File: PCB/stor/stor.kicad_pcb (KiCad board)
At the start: 4 copper layers, 22 x 60.5 mm, 55 parts, among them J1 Conn_01x05_Socket, J2 Conn_01x04_Socket, SW1 TS1603-TZ38HBM, SW2 TS1603-TZ38HBM, U1 STM32H723VGT6, U3 USB3300-EZK-TR, U4 TPS62177DQCR, X1 25mhz, X2 32.768k, X3 24mhz

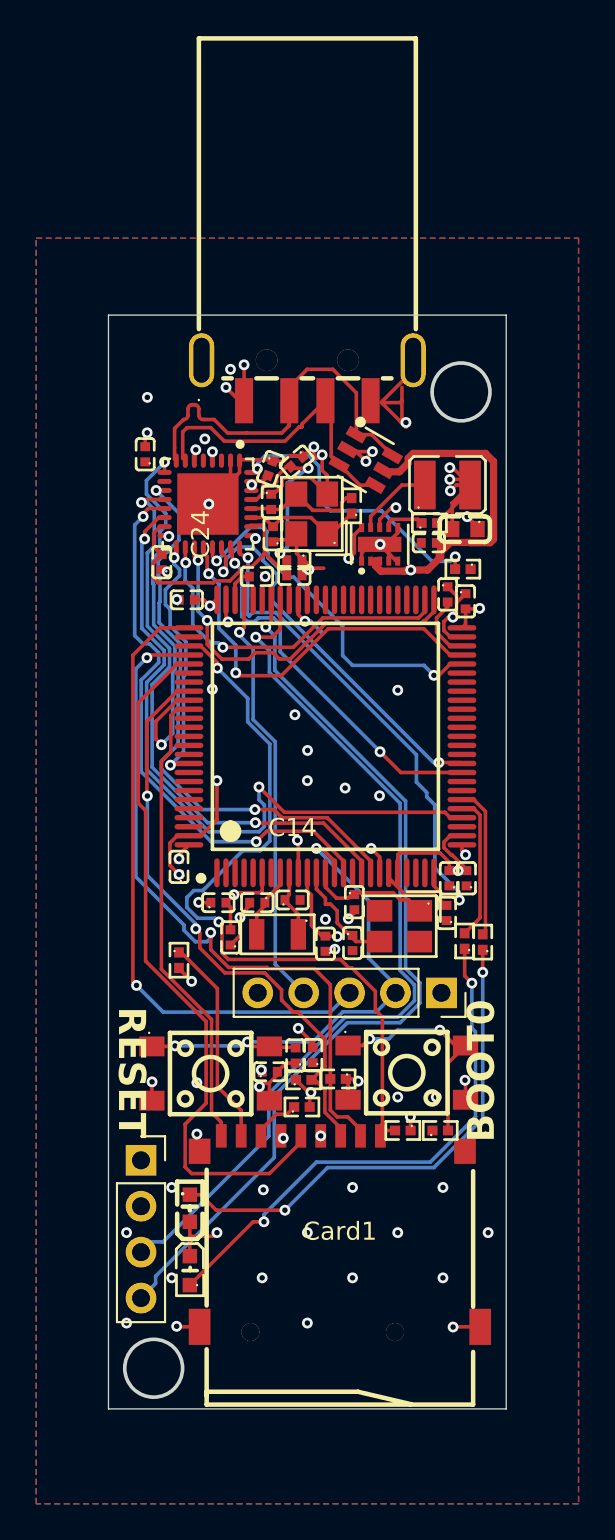
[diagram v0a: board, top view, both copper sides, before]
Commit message: bom opt!!
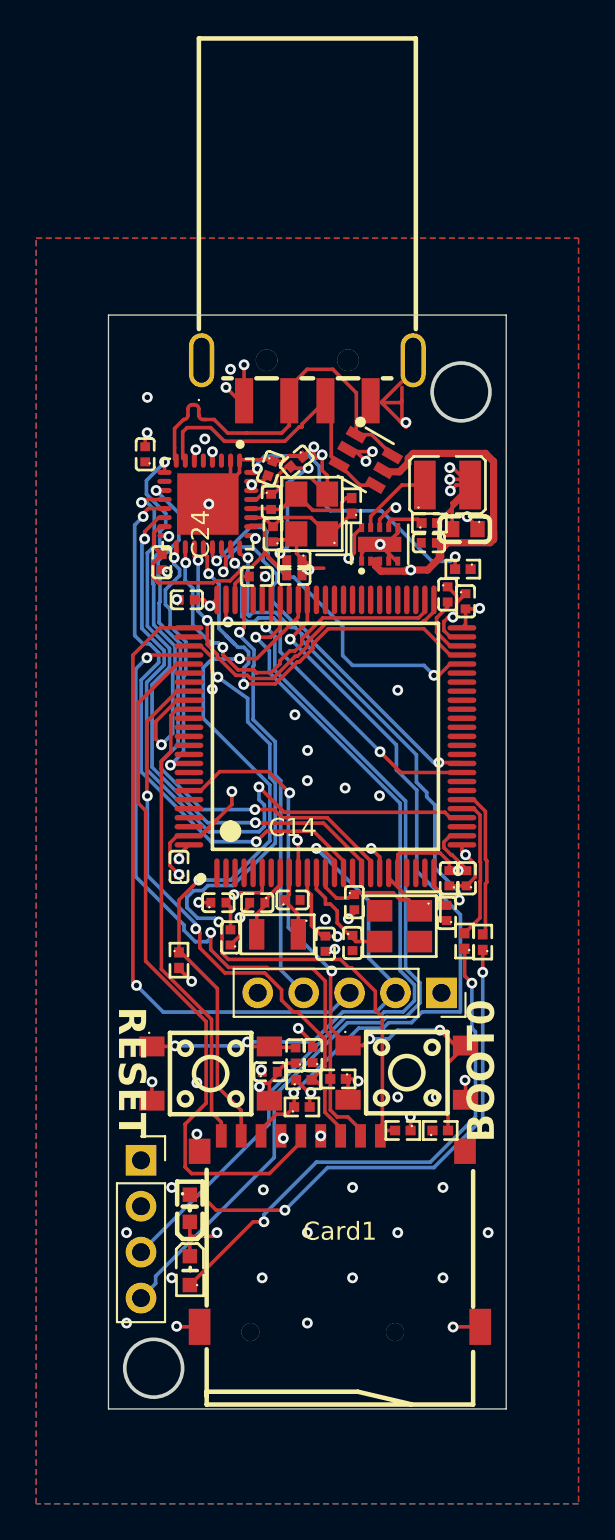
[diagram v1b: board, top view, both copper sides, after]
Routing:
- net /PC8: track 2.35 -> 41.3 mm, vias 0 -> 2
- net /PC9: track 14.3 -> 39.5 mm, vias 1 -> 2
- net /BOOT0: track 11.7 -> 33.7 mm, vias 2 -> 4
- net GND: track 68.5 -> 73.3 mm
- net /PB11: track 21.0 -> 22.7 mm
- net /PB13: track 18.7 -> 20.4 mm
- net /PB12: track 19.9 -> 20.7 mm
- net /PC10: track 40.7 -> 41.3 mm
